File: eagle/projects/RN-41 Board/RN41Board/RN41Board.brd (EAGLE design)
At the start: 38.1 x 16 mm, 18 parts, among them Q1 MOSFET-NCHANNELSMD, U1 BLUETOOTH-RN41, U3 3.3V

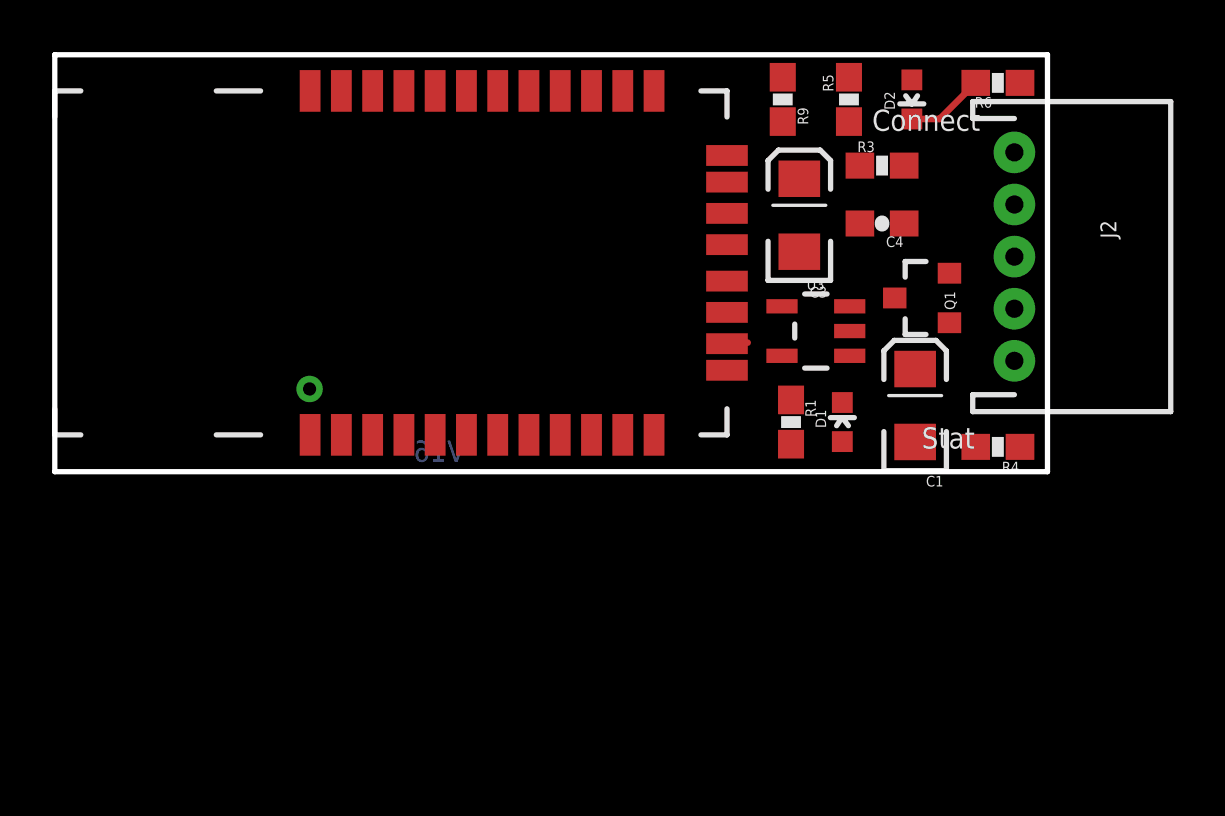
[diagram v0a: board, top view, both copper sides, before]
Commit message: RN41Board UPDATE
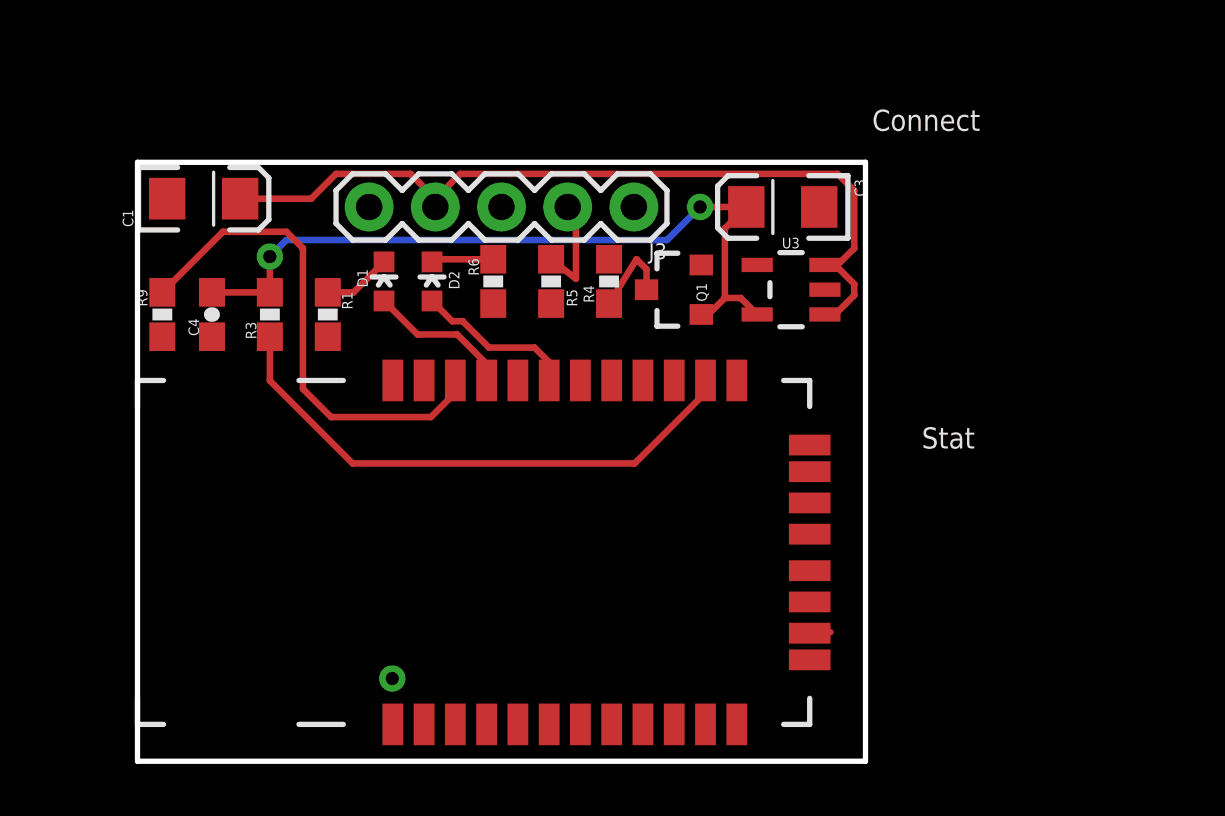
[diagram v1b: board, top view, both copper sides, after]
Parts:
- removed J2: (no value), SparkFun-Connectors:JST-5-PTH
- removed U$1: LOGO-SFENEW, SparkFun:SFE-NEW-WEBLOGO
- added J3: (no value), SparkFun-Connectors:1X05
- moved C1 28.4 mm to (5.71, 10.5), turned to 0 degrees
- moved C4 26.0 mm to (6.03, 6.03), turned to 270 degrees
- moved R9 25.2 mm to (4.13, 6.03), turned to 90 degrees
- moved R3 24.2 mm to (8.26, 6.03), turned to 270 degrees
- moved R6 20.8 mm to (16.8, 7.30), turned to 270 degrees
- moved D2 19.7 mm to (14.5, 7.30), turned to 0 degrees
- moved D1 18.4 mm to (12.6, 7.30)
- moved R1 18.3 mm to (10.5, 6.03)
- moved R4 16.2 mm to (21.3, 7.30), turned to 270 degrees
- moved R5 13.4 mm to (19.1, 7.30), turned to 90 degrees
- moved U1 11.6 mm to (19.6, -3.10)
- moved Q1 9.53 mm to (23.8, 6.99)
- moved U3 1.85 mm to (28.3, 6.99)
- moved C3 0.71 mm to (27.9, 10.2), turned to 180 degrees
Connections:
- net GND: now also J3.5; no longer J2.5
- net PIO2: now also J3.1; no longer J2.1
- net RX_5V: now also J3.2; no longer J2.2
- net TX_5V: now also J3.3; no longer J2.3
- net VCC: now also J3.4; no longer J2.4
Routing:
- net VCC: track 0.00 -> 32.2 mm
- net 3.3V: track 0.00 -> 29.2 mm, vias 0 -> 2
- net TX: track 0.00 -> 21.3 mm
- net PIO4: track 0.01 -> 19.2 mm
- net PIO2: track 0.00 -> 6.17 mm
- net N$1: track 0.00 -> 5.57 mm
- net RX_5V: track 0.00 -> 4.10 mm
- net TX_5V: track 0.00 -> 3.33 mm
- net D1: track 0.00 -> 2.64 mm
- net D2: track 3.03 -> 2.39 mm
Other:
- board size 38.1 x 16 mm -> 27.9 x 23 mm
- board text removed: "BlueSMiRF"
- board text removed: "CTS"
- board text removed: "CTS-I"
- board text removed: "GND"
- board text removed: "Gold"
- board text removed: "HID"
- board text removed: "PIO4"
- board text removed: "RTS"
- board text removed: "RTS-O"
- board text removed: "RX-I"
- board text removed: "Silver"
- board text removed: "TX-O"
- board text removed: "V16"
- board text removed: "VCC"
